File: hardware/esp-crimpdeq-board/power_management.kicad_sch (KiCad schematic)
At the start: 34 parts, among them J1 USB4105-GF-A, Q1 DMG3415U, U3 REF35330QDBVR, U4 MCP1640Bx-xMC, U6 MCP73831T-2ACI/OT

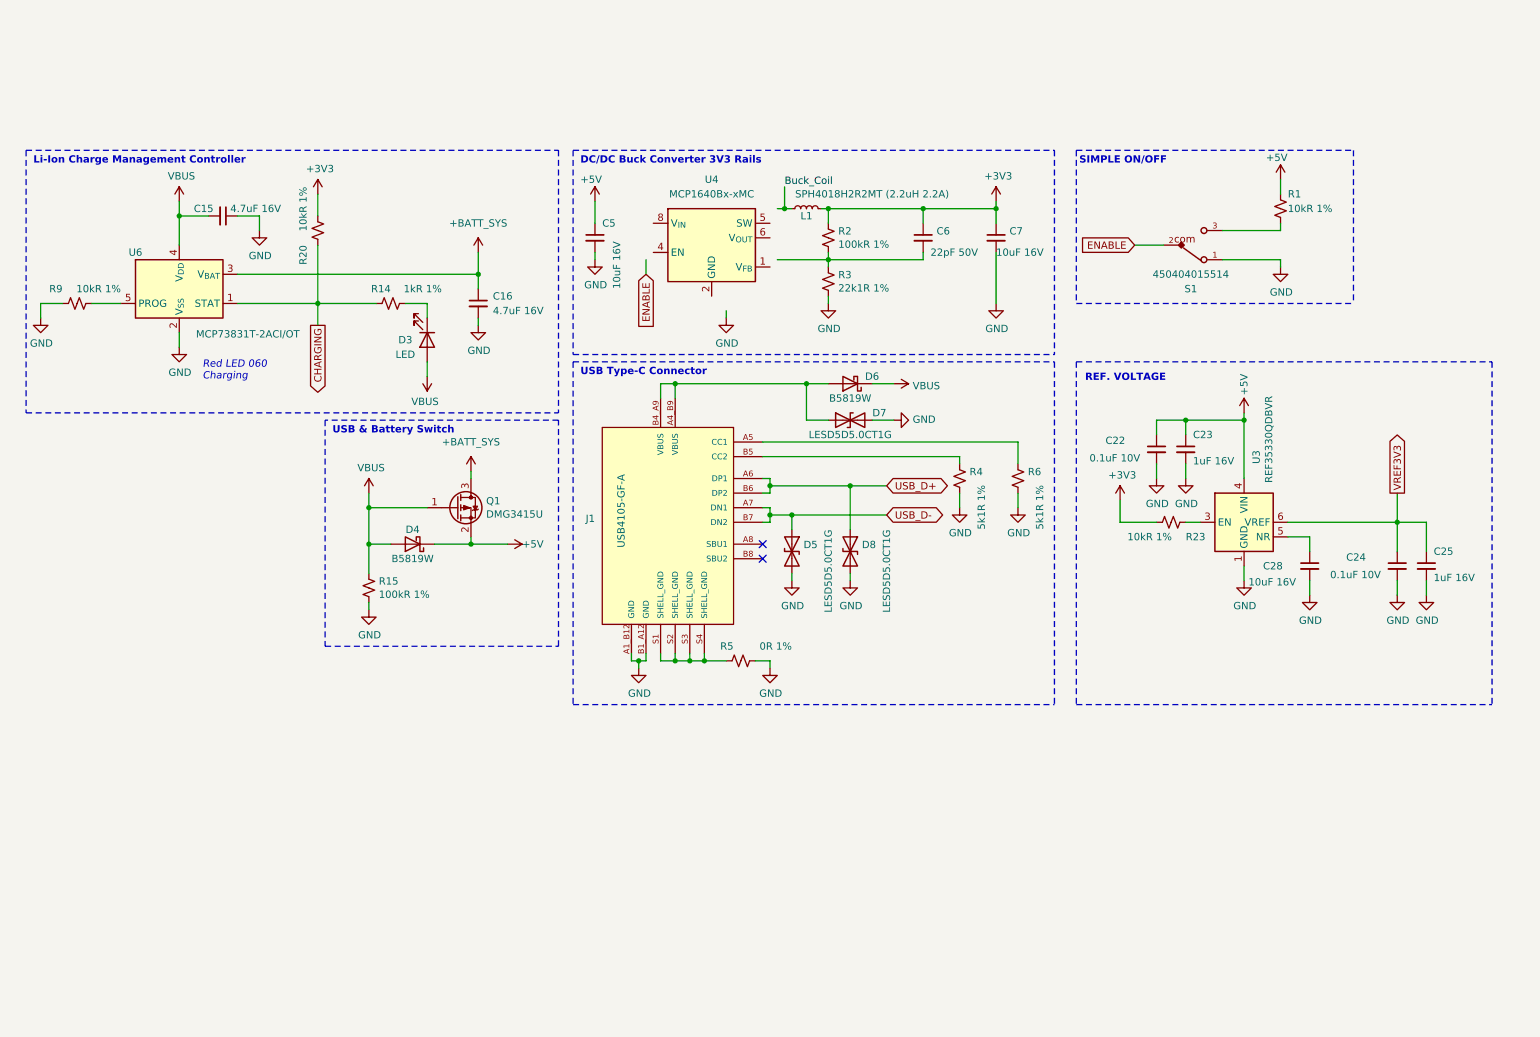
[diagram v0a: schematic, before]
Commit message: Pending
Pending
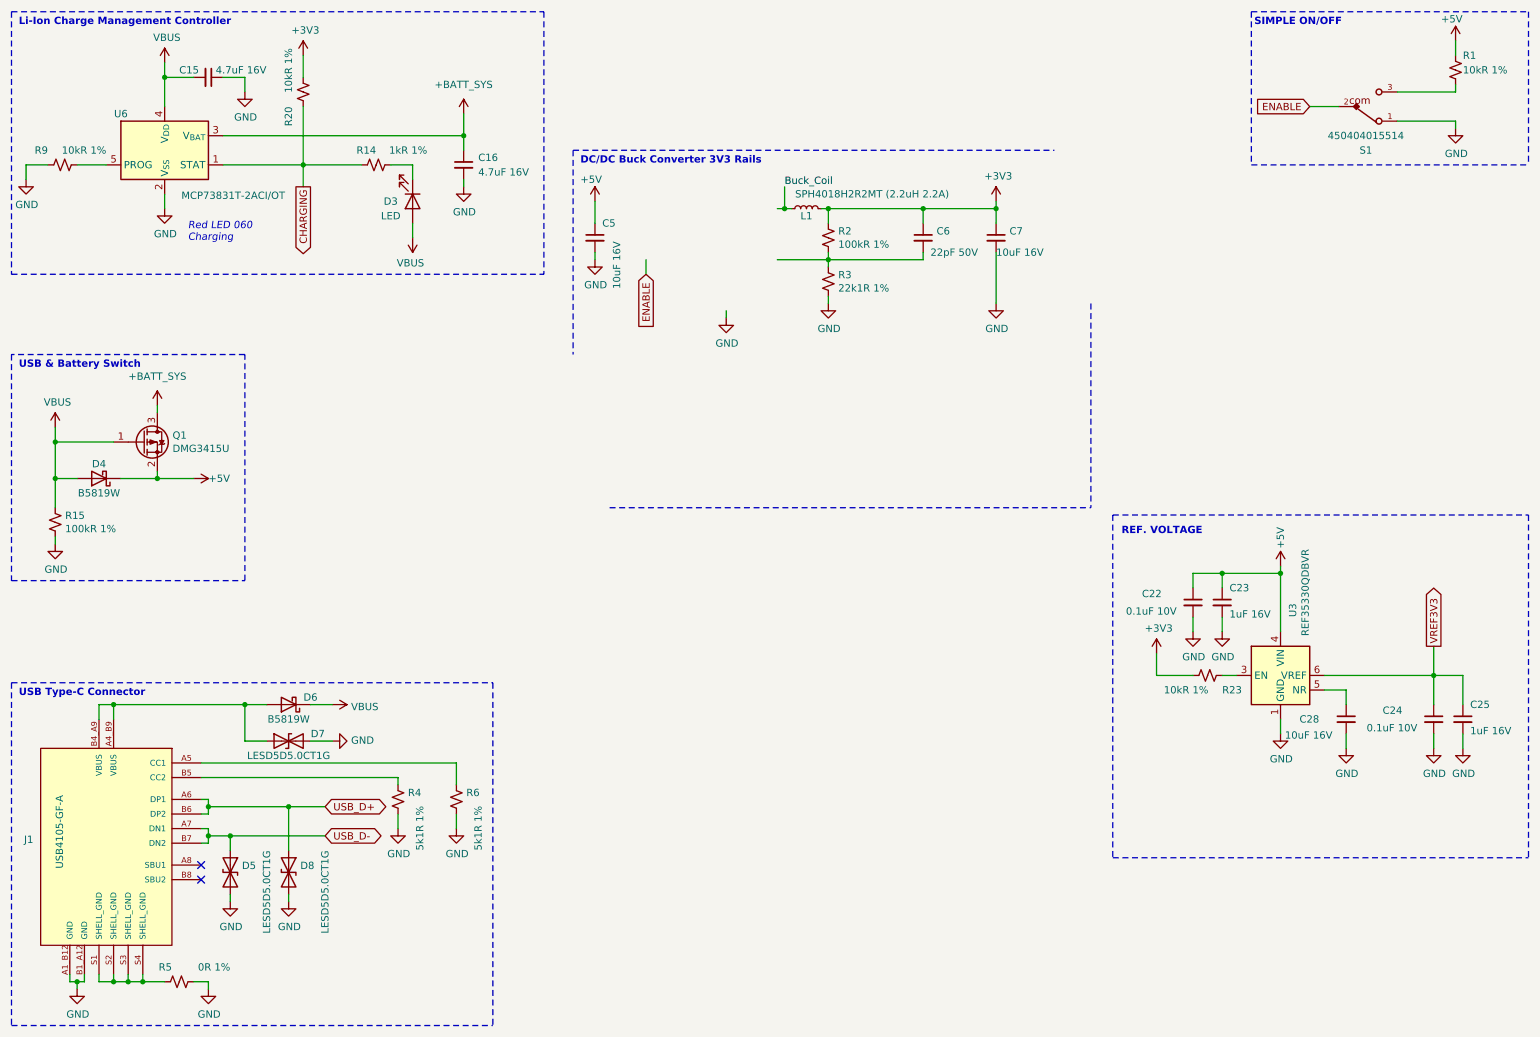
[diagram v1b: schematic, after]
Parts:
- removed U4: MCP1640Bx-xMC, Package_DFN_QFN:DFN-8-1EP_3x2mm_P0.5mm_EP1.75x1.45mm, symbol Regulator_Switching:MCP1640Bx-xMC
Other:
- moved on the sheet: C15, C16, C22, C23, C24, C25, C28, D3, D4, D5, D6, D7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
